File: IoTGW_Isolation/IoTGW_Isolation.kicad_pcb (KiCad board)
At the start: 2 copper layers, 7 parts, among them U2 HCPL-0600, U3 TLE2426xD, U4 VO2630, U5 TEA1-0505, U6 ISO1452BDWR, U7 PC817, U8 PC817

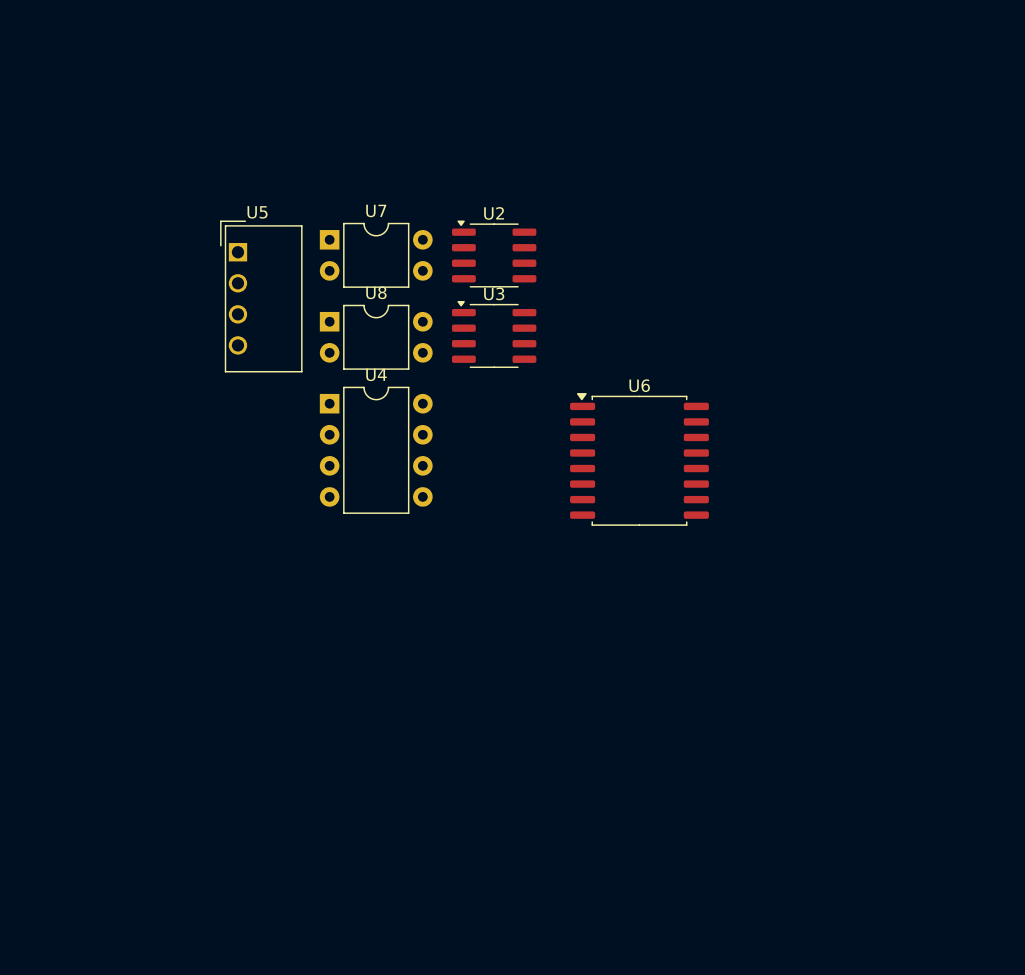
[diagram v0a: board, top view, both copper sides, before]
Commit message: footprints + pcb
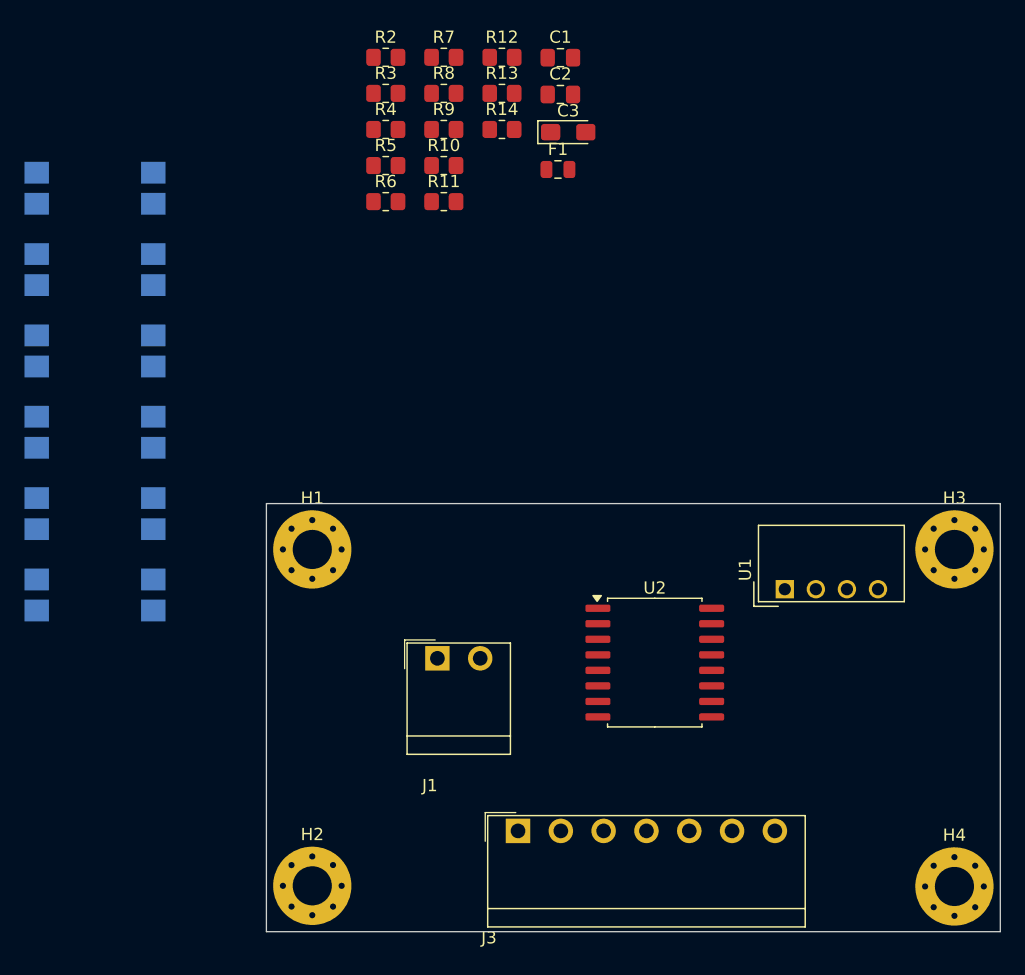
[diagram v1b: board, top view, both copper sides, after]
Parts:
- added C1: 100nF, Capacitor_SMD:C_0805_2012Metric_Pad1.18x1.45mm_HandSolder, F.Cu at (139.0, 53.5)
- added C2: 100nF, Capacitor_SMD:C_0805_2012Metric_Pad1.18x1.45mm_HandSolder, F.Cu at (139.0, 56.6)
- added C3: 10uF, Capacitor_Tantalum_SMD:CP_EIA-3216-18_Kemet-A_Pad1.58x1.35mm_HandSolder, F.Cu at (139.7, 59.6)
- added F1: Polyfuse, Fuse:Fuse_0805_2012Metric, F.Cu at (138.8, 62.7)
- added H1: M3, MountingHole:MountingHole_3.2mm_M3_Pad_Via, F.Cu at (118.8, 93.8)
- added H2: M3, MountingHole:MountingHole_3.2mm_M3_Pad_Via, F.Cu at (118.8, 121.2)
- added H3: M3, MountingHole:MountingHole_3.2mm_M3_Pad_Via, F.Cu at (171.2, 93.8)
- added H4: M3, MountingHole:MountingHole_3.2mm_M3_Pad_Via, F.Cu at (171.2, 121.3)
- added J1: Molex 39502-1002, IoTGW:Molex_2pin_3.50, F.Cu at (126.5, 110.5)
- added J3: Molex 39502-1007, IoTGW:Molex_7pin_3.50, F.Cu at (133.1, 124.6)
- added R10: 200R, Resistor_SMD:R_0805_2012Metric_Pad1.20x1.40mm_HandSolder, F.Cu at (129.5, 62.4)
- added R11: 200R, Resistor_SMD:R_0805_2012Metric_Pad1.20x1.40mm_HandSolder, F.Cu at (129.5, 65.3)
- added R12: 10k, Resistor_SMD:R_0805_2012Metric_Pad1.20x1.40mm_HandSolder, F.Cu at (134.3, 53.5)
- added R13: 10k, Resistor_SMD:R_0805_2012Metric_Pad1.20x1.40mm_HandSolder, F.Cu at (134.3, 56.5)
- added R14: 10k, Resistor_SMD:R_0805_2012Metric_Pad1.20x1.40mm_HandSolder, F.Cu at (134.3, 59.4)
- added R2: 120R, Resistor_SMD:R_0805_2012Metric_Pad1.20x1.40mm_HandSolder, F.Cu at (124.8, 53.5)
- added R3: 200R, Resistor_SMD:R_0805_2012Metric_Pad1.20x1.40mm_HandSolder, F.Cu at (124.8, 56.5)
- added R4: 200R, Resistor_SMD:R_0805_2012Metric_Pad1.20x1.40mm_HandSolder, F.Cu at (124.8, 59.4)
- added R5: 200R, Resistor_SMD:R_0805_2012Metric_Pad1.20x1.40mm_HandSolder, F.Cu at (124.8, 62.4)
- added R6: 10k, Resistor_SMD:R_0805_2012Metric_Pad1.20x1.40mm_HandSolder, F.Cu at (124.8, 65.3)
- added R7: 10k, Resistor_SMD:R_0805_2012Metric_Pad1.20x1.40mm_HandSolder, F.Cu at (129.5, 53.5)
- added R8: 10k, Resistor_SMD:R_0805_2012Metric_Pad1.20x1.40mm_HandSolder, F.Cu at (129.5, 56.5)
- added R9: 200R, Resistor_SMD:R_0805_2012Metric_Pad1.20x1.40mm_HandSolder, F.Cu at (129.5, 59.4)
- added U1: TEA1-0505, Converter_DCDC:Converter_DCDC_TRACO_TEA1-xxxx_THT, F.Cu at (157.4, 97.0)
- U2: value HCPL-0600 -> ISO1452BDWR; footprint Package_SO:SOIC-8_3.9x4.9mm_P1.27mm -> Package_SO:SOIC-16W_7.5x10.3mm_P1.27mm
- U3: value TLE2426xD -> LTV-817S; footprint Package_SO:SOIC-8_3.9x4.9mm_P1.27mm -> Package_DIP:SMDIP-4_W9.53mm; moved to B.Cu
- U4: value VO2630 -> LTV-817S; footprint Package_DIP:DIP-8_W7.62mm -> Package_DIP:SMDIP-4_W9.53mm; moved to B.Cu
- U5: value TEA1-0505 -> LTV-817S; footprint Converter_DCDC:Converter_DCDC_TRACO_TEA1-xxxx_THT -> Package_DIP:SMDIP-4_W9.53mm; moved to B.Cu
- U6: value ISO1452BDWR -> LTV-817S; footprint Package_SO:SOIC-16W_7.5x10.3mm_P1.27mm -> Package_DIP:SMDIP-4_W9.53mm; moved to B.Cu
- U7, U8: value PC817 -> LTV-817S; footprint Package_DIP:DIP-4_W7.62mm -> Package_DIP:SMDIP-4_W9.53mm; moved to B.Cu
- moved U6 44.6 mm to (101.0, 84.2), turned to 180 degrees
- moved U2 35.8 mm to (146.8, 103.0)
- moved U3 34.8 mm to (101.0, 64.2), turned to 180 degrees
- moved U7 29.5 mm to (101.0, 90.8), turned to 180 degrees
- moved U8 29.4 mm to (101.0, 97.5), turned to 180 degrees
- moved U4 22.1 mm to (101.0, 70.9), turned to 180 degrees
- moved U5 14.2 mm to (101.0, 77.5), turned to 180 degrees
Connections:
- U2 pad 1: unconnected-(U2-NC-Pad1) -> +5V
- U2 pad 2: Net-(U2-A) -> GND
- U2 pad 3: GND -> GPIO_R
- U2 pad 4: (no net) -> GPIO_~{RE}
- U2 pad 5: GND_OUT -> GPIO_DE
- U2 pad 6: unconnected-(U2-VO-Pad6) -> GPIO_D
- U2 pad 8: unconnected-(U2-VCC-Pad8) -> GND
- U3 pad 1: GND1 -> Net-(R3-Pad1)
- U3 pad 3: VCC -> GND_OUT
- U3 pad 4: unconnected-(U3-NC-Pad4) -> GPIO_EXT_0
- U4 pad 1: unconnected-(U4-A1-Pad1) -> Net-(R4-Pad1)
- U4 pad 2: unconnected-(U4-C1-Pad2) -> GND
- U4 pad 3: unconnected-(U4-C2-Pad3) -> GND_OUT
- U4 pad 4: unconnected-(U4-A2-Pad4) -> GPIO_EXT_1
- U5 pad 1: GND -> Net-(R5-Pad1)
- U5 pad 2: +5V -> GND
- U5 pad 4: +5V_OUT -> GPIO_EXT_2
- U6 pad 1: +5V -> Net-(R9-Pad1)
- U6 pad 2: GND -> GND_OUT
- U6 pad 3: GPIO_ -> GND
- U6 pad 4: GPIO_~{RE} -> GPIO_OPTO_0
- U7 pad 2: GND -> GND_OUT
- U7 pad 3: GND_OUT -> GND
- U7 pad 4: GPIO_EXT_0 -> GPIO_OPTO_1
- U8 pad 4: GPIO_0 -> GPIO_OPTO_2
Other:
- board outline added: 60 x 35 mm
- copper layers 2 -> 4
